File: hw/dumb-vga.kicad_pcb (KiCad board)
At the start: 2 copper layers, 62.2 x 83.8 mm, 26 parts, among them IC1 74HC590N, IC2 74HC590N, IC3 74HC590N, IC4 74HC574N, P1 CONN_01X03, P2 CONN_01X03, P3 CONN_01X03, U1 A29040C, X1 VGAF

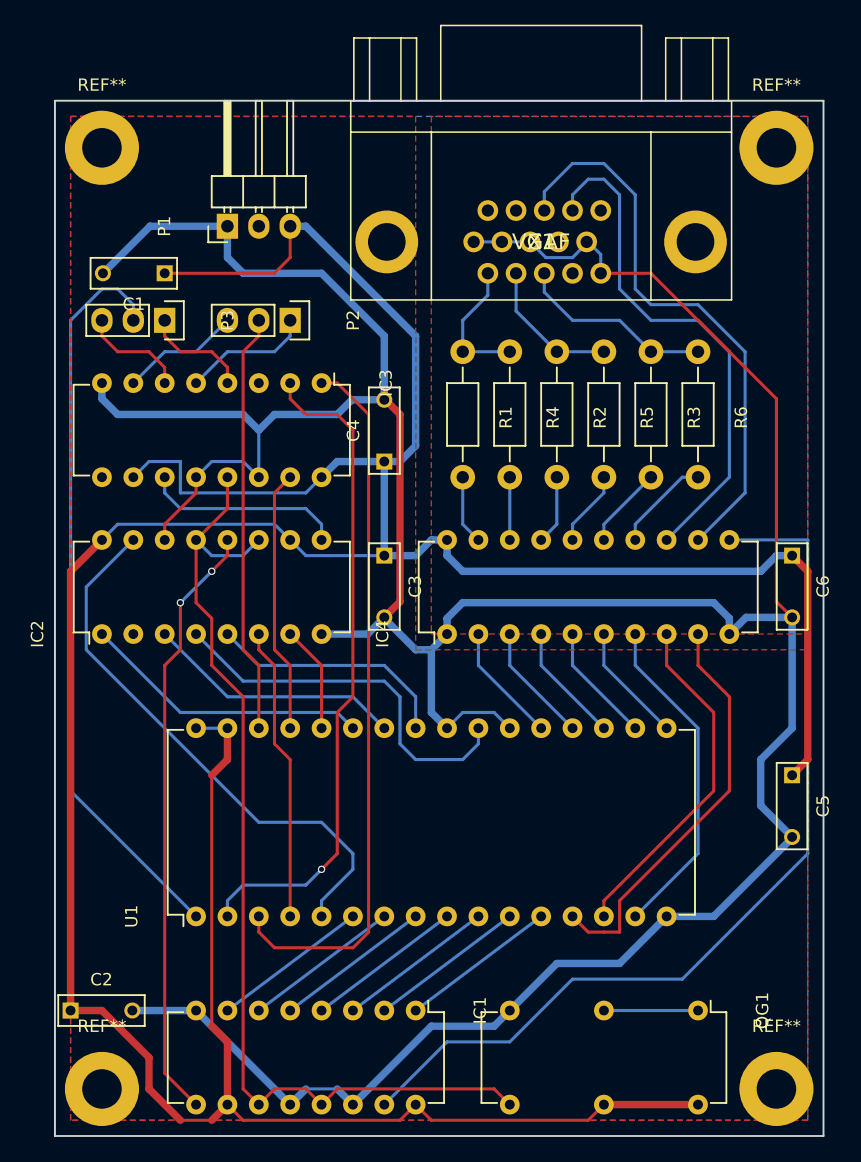
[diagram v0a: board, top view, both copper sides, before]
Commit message: Bumping schematic version number, labelling up PCB
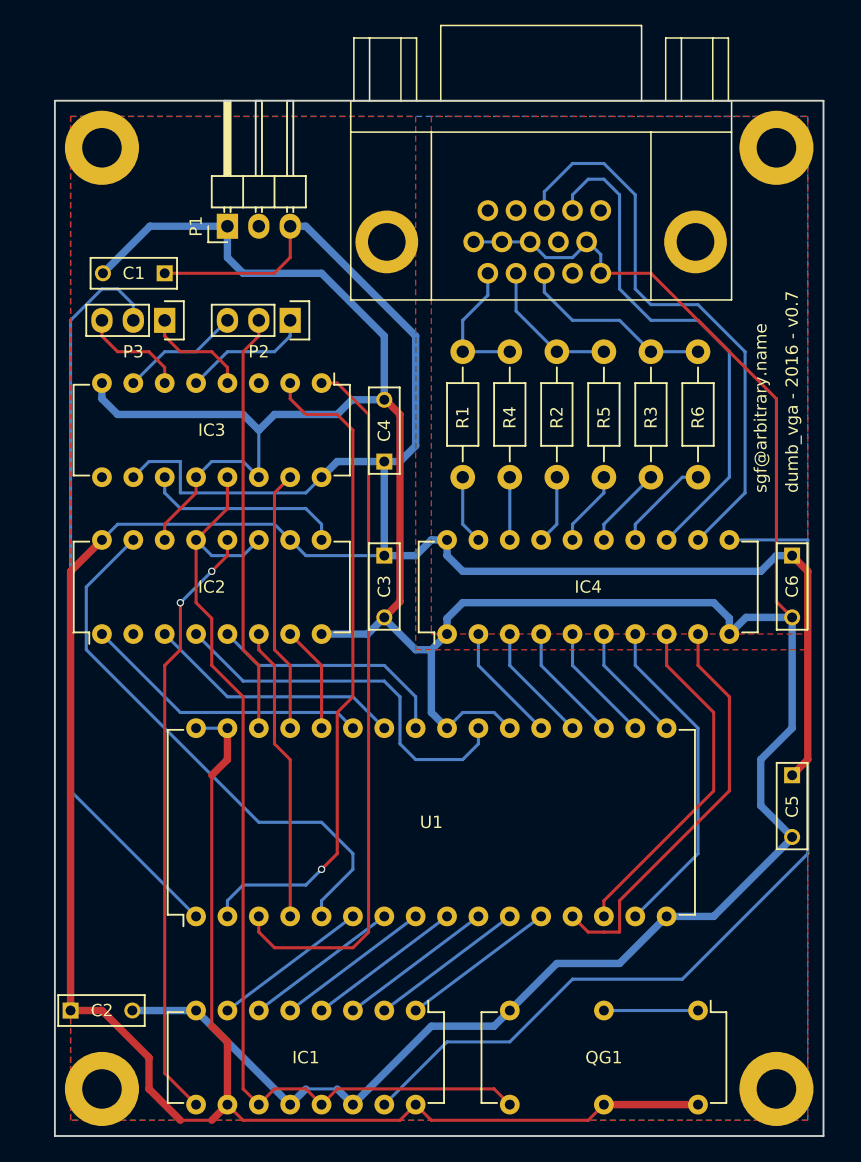
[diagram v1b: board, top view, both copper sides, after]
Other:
- board text added: "dumb_vga - 2016 - v0.7"
- board text added: "sgf@arbitrary.name"
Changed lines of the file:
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@@
     (links 96)
     (no_connects 0)
-    (area 104.064999 32.944999 166.445001 116.915001)
+    (area 96.135475 26.663039 176.914525 119.085)
     (thickness 1.6)
-    (drawings 4)
+    (drawings 6)
     (tracks 333)
     (zones 0)
@@
   )
   (page A4)
+  (title_block
+    (title "Dumb VGA")
+    (rev v0.7)
+    (comment 1 "Simple circuit to generate VGA-like signal")
+  )
   (layers
-    (0 F.Cu signal hide)
+    (0 F.Cu signal)
     (31 B.Cu signal)
     (32 B.Adhes user)
@@
     (descr "14-lead dip package, row spacing 7.62 mm (300 mils)")
     (tags "dil dip 2.54 300")
-    (fp_text reference QG1 (at 0 -5.22 270) (layer F.SilkS)
+    (fp_text reference QG1 (at 3.81 7.62 360) (layer F.SilkS)
       (effects (font (size 1 1) (thickness 0.15)))
     )
@@
   (module Wire_Pads:SolderWirePad_single_2-5mmDrill (layer F.Cu)
     (at 162.56 113.03)
-    (fp_text reference REF** (at 0 -5.08) (layer F.SilkS)
+    (fp_text reference REF** (at 0 -5.08) (layer F.SilkS) hide
       (effects (font (size 1 1) (thickness 0.15)))
     )
@@
   (module Wire_Pads:SolderWirePad_single_2-5mmDrill (layer F.Cu)
     (at 107.95 113.03)
-    (fp_text reference REF** (at 0 -5.08) (layer F.SilkS)
+    (fp_text reference REF** (at 0 -5.08) (layer F.SilkS) hide
       (effects (font (size 1 1) (thickness 0.15)))
     )
@@
   (module Wire_Pads:SolderWirePad_single_2-5mmDrill (layer F.Cu)
     (at 107.95 36.83)
-    (fp_text reference REF** (at 0 -5.08) (layer F.SilkS)
+    (fp_text reference REF** (at 0 -5.08) (layer F.SilkS) hide
       (effects (font (size 1 1) (thickness 0.15)))
     )
@@
     (at 143.51 44.45)
     (attr virtual)
-    (fp_text reference X1 (at 0 0) (layer F.SilkS)
+    (fp_text reference X1 (at 0 0) (layer F.SilkS) hide
       (effects (font (thickness 0.15)))
     )
-    (fp_text value VGAF (at 0 0) (layer F.SilkS)
+    (fp_text value VGAF (at 0 0) (layer F.SilkS) hide
       (effects (font (thickness 0.15)))
     )
@@
     (descr "Film Capacitor Length 7mm x Width 2.5mm, Pitch 5mm")
     (tags Capacitor)
-    (fp_text reference C1 (at 2.5 -2.5 180) (layer F.SilkS)
+    (fp_text reference C1 (at 2.5 0 180) (layer F.SilkS)
       (effects (font (size 1 1) (thickness 0.15)))
     )
@@
     (descr "16-lead dip package, row spacing 7.62 mm (300 mils)")
     (tags "dil dip 2.54 300")
-    (fp_text reference IC1 (at 0 -5.22 270) (layer F.SilkS)
+    (fp_text reference IC1 (at 3.81 8.89 360) (layer F.SilkS)
       (effects (font (size 1 1) (thickness 0.15)))
     )
@@
     (descr "16-lead dip package, row spacing 7.62 mm (300 mils)")
     (tags "dil dip 2.54 300")
-    (fp_text reference IC2 (at 0 -5.22 90) (layer F.SilkS)
+    (fp_text reference IC2 (at 3.81 8.89 180) (layer F.SilkS)
       (effects (font (size 1 1) (thickness 0.15)))
     )
@@
     (descr "16-lead dip package, row spacing 7.62 mm (300 mils)")
     (tags "dil dip 2.54 300")
-    (fp_text reference IC3 (at 0 -5.22 270) (layer F.SilkS)
+    (fp_text reference IC3 (at 3.81 8.89 360) (layer F.SilkS)
       (effects (font (size 1 1) (thickness 0.15)))
     )
@@
     (descr "20-lead dip package, row spacing 7.62 mm (300 mils)")
     (tags "dil dip 2.54 300")
-    (fp_text reference IC4 (at 0 -5.22 90) (layer F.SilkS)
+    (fp_text reference IC4 (at 3.81 11.43 180) (layer F.SilkS)
       (effects (font (size 1 1) (thickness 0.15)))
     )
@@
     (descr "Resistor, Axial,  RM 10mm, 1/3W,")
     (tags "Resistor, Axial, RM 10mm, 1/3W,")
-    (fp_text reference R1 (at 0.24892 -3.50012 270) (layer F.SilkS)
+    (fp_text reference R1 (at 0.24892 0 270) (layer F.SilkS)
       (effects (font (size 1 1) (thickness 0.15)))
     )
@@
     (descr "Resistor, Axial,  RM 10mm, 1/3W,")
     (tags "Resistor, Axial, RM 10mm, 1/3W,")
-    (fp_text reference R2 (at 0.24892 -3.50012 270) (layer F.SilkS)
+    (fp_text reference R2 (at 0.24892 0 270) (layer F.SilkS)
       (effects (font (size 1 1) (thickness 0.15)))
     )
@@
     (descr "Resistor, Axial,  RM 10mm, 1/3W,")
     (tags "Resistor, Axial, RM 10mm, 1/3W,")
-    (fp_text reference R3 (at 0.24892 -3.50012 270) (layer F.SilkS)
+    (fp_text reference R3 (at 0.24892 0 270) (layer F.SilkS)
       (effects (font (size 1 1) (thickness 0.15)))
     )
@@
     (descr "Resistor, Axial,  RM 10mm, 1/3W,")
     (tags "Resistor, Axial, RM 10mm, 1/3W,")
-    (fp_text reference R4 (at 0.24892 -3.50012 270) (layer F.SilkS)
+    (fp_text reference R4 (at 0.24892 0 270) (layer F.SilkS)
       (effects (font (size 1 1) (thickness 0.15)))
     )
@@
     (descr "Resistor, Axial,  RM 10mm, 1/3W,")
     (tags "Resistor, Axial, RM 10mm, 1/3W,")
-    (fp_text reference R5 (at 0.24892 -3.50012 270) (layer F.SilkS)
+    (fp_text reference R5 (at 0.24892 0 270) (layer F.SilkS)
       (effects (font (size 1 1) (thickness 0.15)))
     )
@@
     (descr "Resistor, Axial,  RM 10mm, 1/3W,")
     (tags "Resistor, Axial, RM 10mm, 1/3W,")
-    (fp_text reference R6 (at 0.24892 -3.50012 270) (layer F.SilkS)
+    (fp_text reference R6 (at 0.24892 0 270) (layer F.SilkS)
       (effects (font (size 1 1) (thickness 0.15)))
     )
@@
     (descr "32-lead dip package, row spacing 15.24 mm (600 mils)")
     (tags "dil dip 2.54 600")
-    (fp_text reference U1 (at 0 -5.22 90) (layer F.SilkS)
+    (fp_text reference U1 (at 7.62 19.05 180) (layer F.SilkS)
       (effects (font (size 1 1) (thickness 0.15)))
     )
@@
     (descr "Film Capacitor Length 7mm x Width 2.5mm, Pitch 5mm")
     (tags Capacitor)
-    (fp_text reference C2 (at 2.5 -2.5) (layer F.SilkS)
+    (fp_text reference C2 (at 2.54 0) (layer F.SilkS)
       (effects (font (size 1 1) (thickness 0.15)))
     )
@@
     (descr "Film Capacitor Length 7mm x Width 2.5mm, Pitch 5mm")
     (tags Capacitor)
-    (fp_text reference C3 (at 2.5 -2.5 270) (layer F.SilkS)
+    (fp_text reference C3 (at 2.5 0 270) (layer F.SilkS)
       (effects (font (size 1 1) (thickness 0.15)))
     )
@@
     (descr "Film Capacitor Length 7mm x Width 2.5mm, Pitch 5mm")
     (tags Capacitor)
-    (fp_text reference C4 (at 2.5 -2.5 90) (layer F.SilkS)
+    (fp_text reference C4 (at 2.5 0 90) (layer F.SilkS)
       (effects (font (size 1 1) (thickness 0.15)))
     )
@@
     (descr "Film Capacitor Length 7mm x Width 2.5mm, Pitch 5mm")
     (tags Capacitor)
-    (fp_text reference C5 (at 2.5 -2.5 270) (layer F.SilkS)
+    (fp_text reference C5 (at 2.54 0 270) (layer F.SilkS)
       (effects (font (size 1 1) (thickness 0.15)))
     )
@@
     (descr "Film Capacitor Length 7mm x Width 2.5mm, Pitch 5mm")
     (tags Capacitor)
-    (fp_text reference C6 (at 2.5 -2.5 270) (layer F.SilkS)
+    (fp_text reference C6 (at 2.5 0 270) (layer F.SilkS)
       (effects (font (size 1 1) (thickness 0.15)))
     )
@@
     (descr "Through hole pin header")
     (tags "pin header")
-    (fp_text reference P2 (at 0 -5.1 270) (layer F.SilkS)
+    (fp_text reference P2 (at 2.54 2.54 360) (layer F.SilkS)
       (effects (font (size 1 1) (thickness 0.15)))
     )
@@
     (descr "Through hole pin header")
     (tags "pin header")
-    (fp_text reference P3 (at 0 -5.1 270) (layer F.SilkS)
+    (fp_text reference P3 (at 2.54 2.54 360) (layer F.SilkS)
       (effects (font (size 1 1) (thickness 0.15)))
     )
@@
   (module Wire_Pads:SolderWirePad_single_2-5mmDrill (layer F.Cu)
     (at 162.56 36.83)
-    (fp_text reference REF** (at 0 -5.08) (layer F.SilkS)
+    (fp_text reference REF** (at 0 -5.08) (layer F.SilkS) hide
       (effects (font (size 1 1) (thickness 0.15)))
     )
@@
     (descr "Through hole pin header")
     (tags "pin header")
-    (fp_text reference P1 (at 0 -5.1 90) (layer F.SilkS)
+    (fp_text reference P1 (at 0 -2.54 90) (layer F.SilkS)
       (effects (font (size 1 1) (thickness 0.15)))
     )
@@
     )
   )
+  (gr_text "dumb_vga - 2016 - v0.7" (at 163.83 64.77 90) (layer F.SilkS)
+    (effects (font (size 1 1) (thickness 0.15)) (justify left))
+  )
+  (gr_text sgf@arbitrary.name (at 161.29 64.77 90) (layer F.SilkS)
+    (effects (font (size 1 1) (thickness 0.15)) (justify left))
+  )
   (gr_line (start 104.14 116.84) (end 104.14 33.02) (angle 90) (layer Edge.Cuts) (width 0.15))
